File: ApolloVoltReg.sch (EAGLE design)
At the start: 27 parts, among them IC2 TL084D, J1 SSM-108-L-DV-BE-K-APOLLO, U1 TEXAS_INSTRUMENTS_PTH04070WAD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, U2 ACS712ELCTR-05B-T

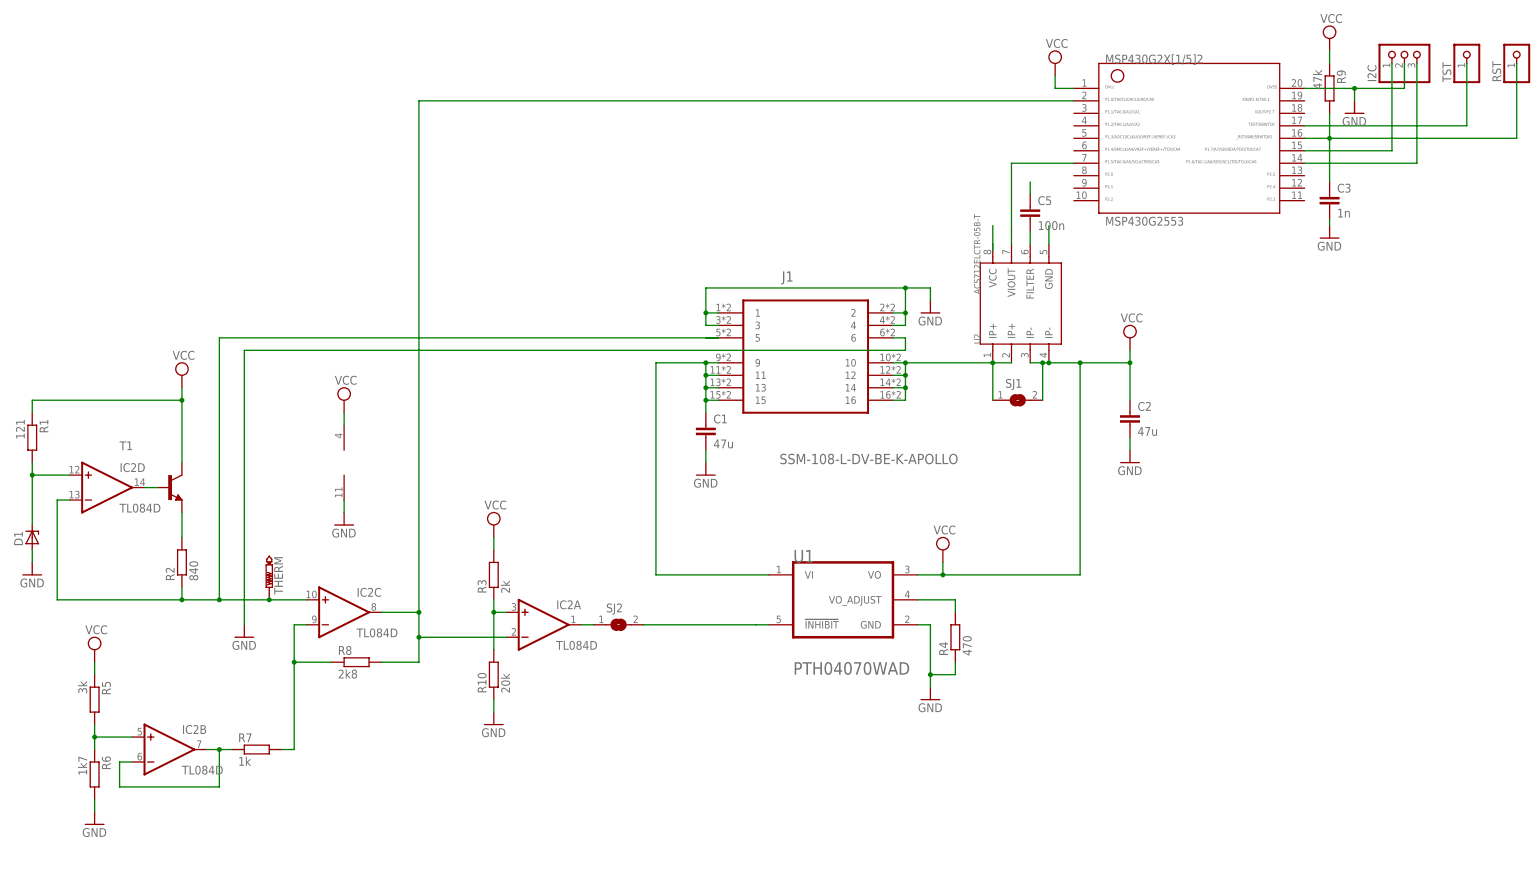
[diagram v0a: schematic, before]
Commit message: adding pic
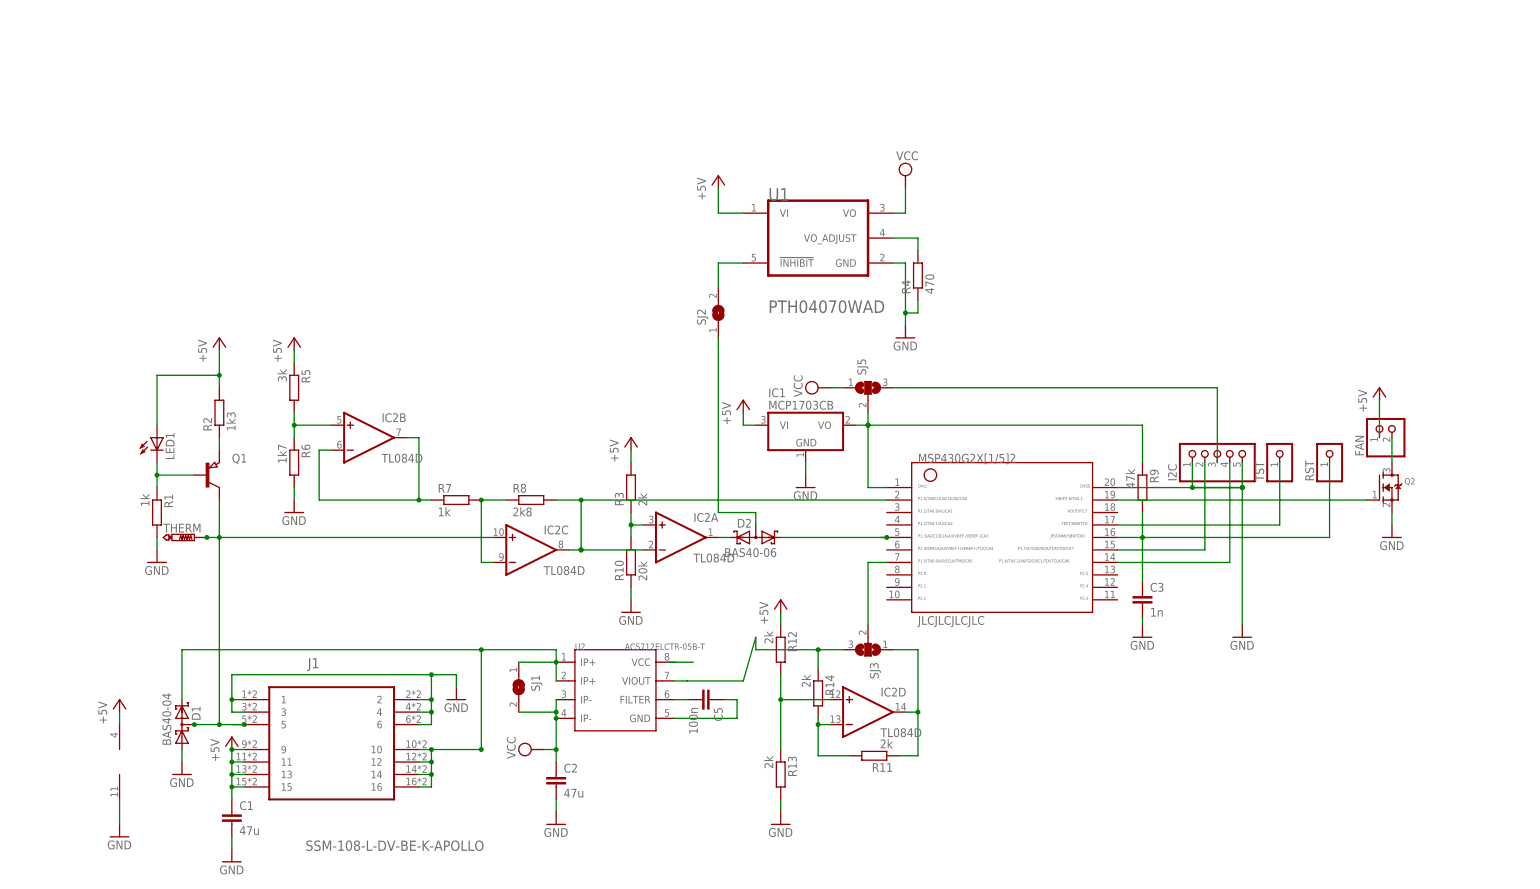
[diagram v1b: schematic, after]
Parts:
- removed MSP430G2553: G2X[1/5]2---N20, TI_MSP430_v16:G2X[1/5]2---N20
- removed T1: (no value), transistor:-NPN-SOT23-EBC
- added D2: BAS40-06, diode:BAS40-06
- added FAN: (no value), pinhead:PINHD-1X2
- added IC1: MCP1703CB, linear:MCP1703CB
- added JLCJLCJLCJLC: G2X[1/5]2---N20, TI_MSP430_v16:G2X[1/5]2---N20
- added LED1: (no value), adafruit:LED3MM
- added Q1: (no value), semicon-smd-ipc:PNP-TRANSISTOR_SOT23
- added Q2: (no value), adafruit:MOSFET-NREFLOW
- added R11, R12, R13: 2k, resistor:R-EU_R0805
- added R14: 2k, resistor:R-EU_R0603
- added SJ3, SJ5: (no value), jumper:SJ2W
- C1, C2: device eagle-ltspice:CC1206 -> eagle-ltspice:CC1210
- D1: value (none) -> BAS40-04; device diode:ZENER-DIODESOD80C -> diode:BAS40-04
- I2C: device adafruit:PINHD-1X3 -> pinhead:PINHD-1X5
- R1: value 121 -> 1k; device resistor:R-EU_R0603 -> resistor:R-EU_R0805
- R10, R3, R4, R5, R6, R7, R8: device resistor:R-EU_R0603 -> resistor:R-EU_R0805
- R2: value 840 -> 1k3; device resistor:R-EU_R0603 -> resistor:R-EU_R0805
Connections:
- new net N$13: IC2D.-IN, R11.2, R14.2
- new net N$14: IC2D.OUT, R11.1, SJ3.1
- new net N$15: JLCJLCJLCJLC.7, SJ3.2
- new net N$16: IC1.VO, JLCJLCJLCJLC.1, R9.1, SJ5.2
- new net N$17: D2.K2, IC2A.OUT
- new net N$18: D2.AA, SJ2.1
- new net N$19: FAN.2, Q2.D
- new net N$21: I2C.3, SJ5.3
- new net RST: C3.1, JLCJLCJLCJLC.16, R9.2, RST.1
- net +5V: now also FAN.1, IC1.VI, IC2P.V+, LED1.A, R12.1, R2.2, R3.2, R5.1
- net ACS_OUT: now also R14.1, SJ3.3; no longer MSP430G2553.7
- net CPU: now also D1.C2
- net GND: now also D1.A1, I2C.1, I2C.5, IC1.GND, JLCJLCJLCJLC.20, Q2.S, R1.2, R13.2; no longer D1.A, I2C.2, MSP430G2553.20
- net N$10: now also JLCJLCJLCJLC.17; no longer MSP430G2553.17
- net N$12: now also D2.K1, JLCJLCJLCJLC.5; no longer IC2A.OUT, SJ2.1
- net N$2: now also LED1.C, Q1.B, R1.1; no longer D1.C, IC2D.+IN, R1.2
- net N$3: now also Q1.E, R2.1; no longer IC2D.OUT, T1.B
- net N$4: now also IC2D.+IN, R12.2, R13.1; no longer R2.2, T1.E
- net N$9: now also JLCJLCJLCJLC.19, Q2.G; no longer C3.1, MSP430G2553.16, R9.2, RST.1
- net SCL: now also I2C.4, JLCJLCJLCJLC.14; no longer I2C.3, MSP430G2553.14
- net SDA: now also I2C.2, JLCJLCJLCJLC.15; no longer I2C.1, MSP430G2553.15
- net TEMPSENS: now also JLCJLCJLCJLC.2; no longer MSP430G2553.2
- net THERM1: now also D1.C1A2, Q1.C; no longer IC2D.-IN, R2.1
- net VCC: now also SJ5.1; no longer IC2P.V+, MSP430G2553.1, R1.1, R3.2, R5.1, R9.1, T1.C
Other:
- moved on the sheet: C1, C2, C3, C5, IC2A, IC2B, IC2C, IC2D, J1, R1, R10, R2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
